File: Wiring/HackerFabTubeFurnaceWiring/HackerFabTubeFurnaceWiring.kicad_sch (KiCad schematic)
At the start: 11 parts

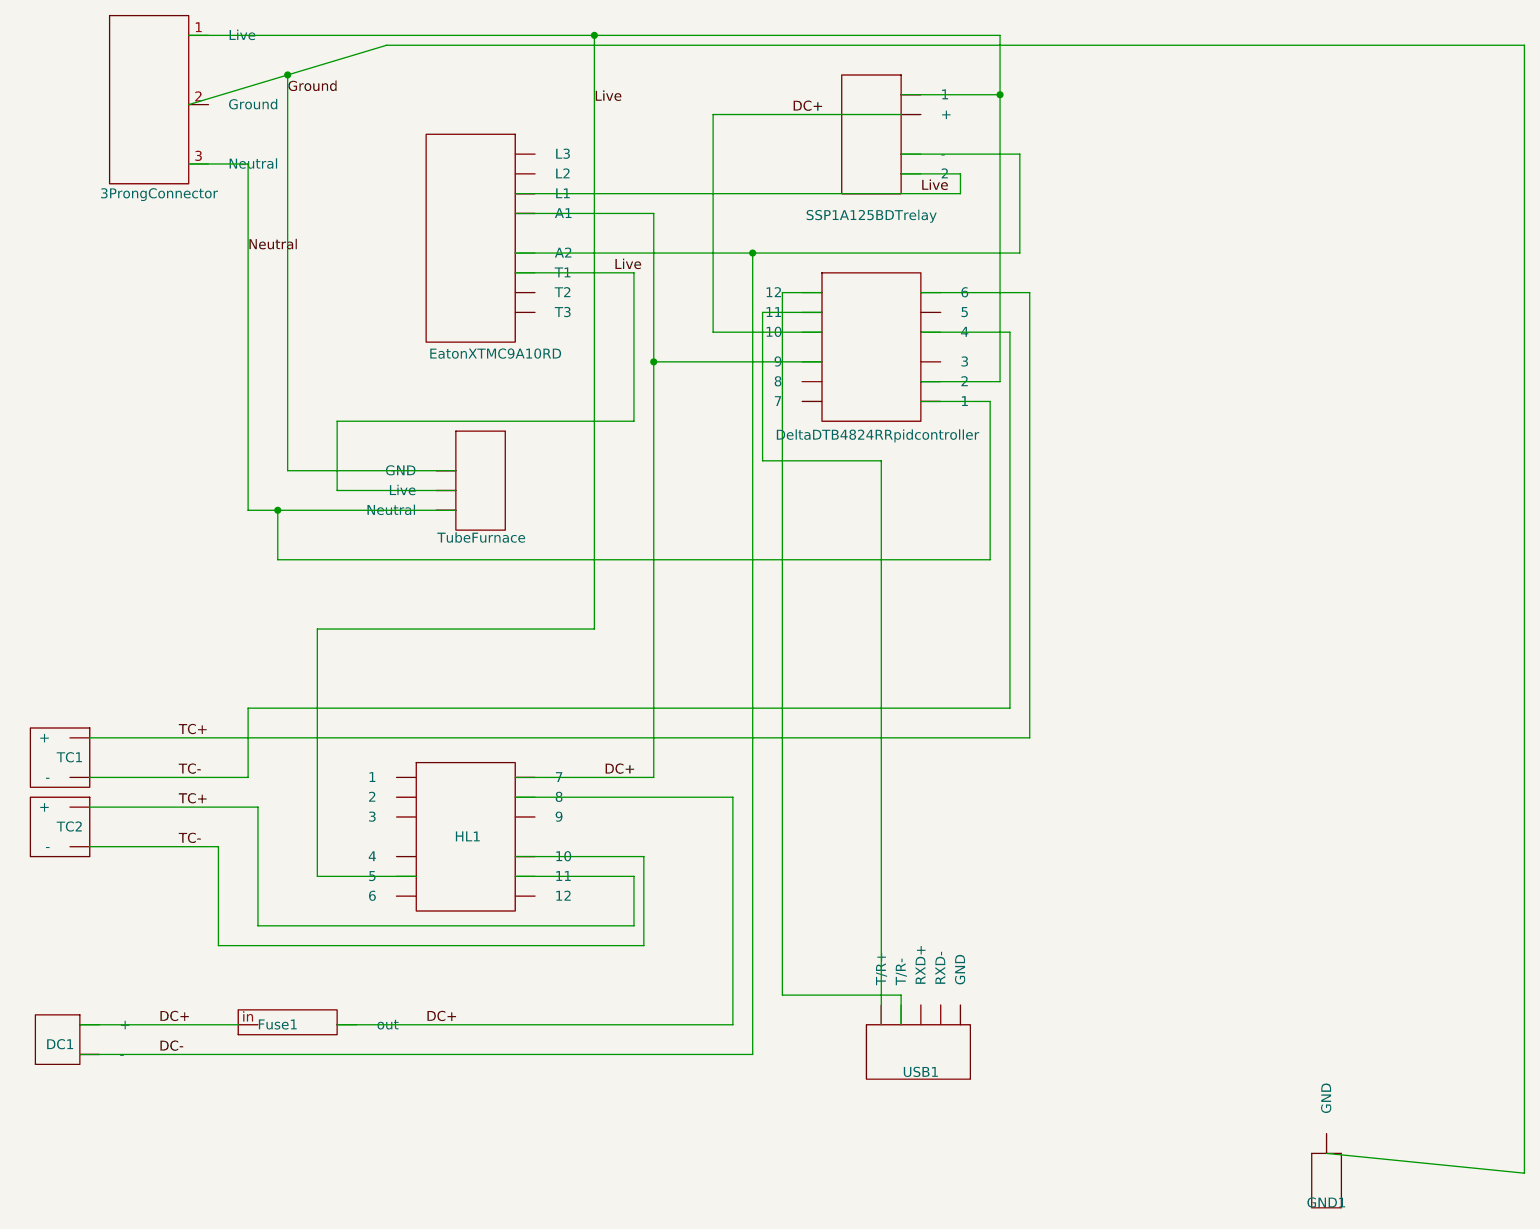
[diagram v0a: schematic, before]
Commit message: Adjustments to Schematic
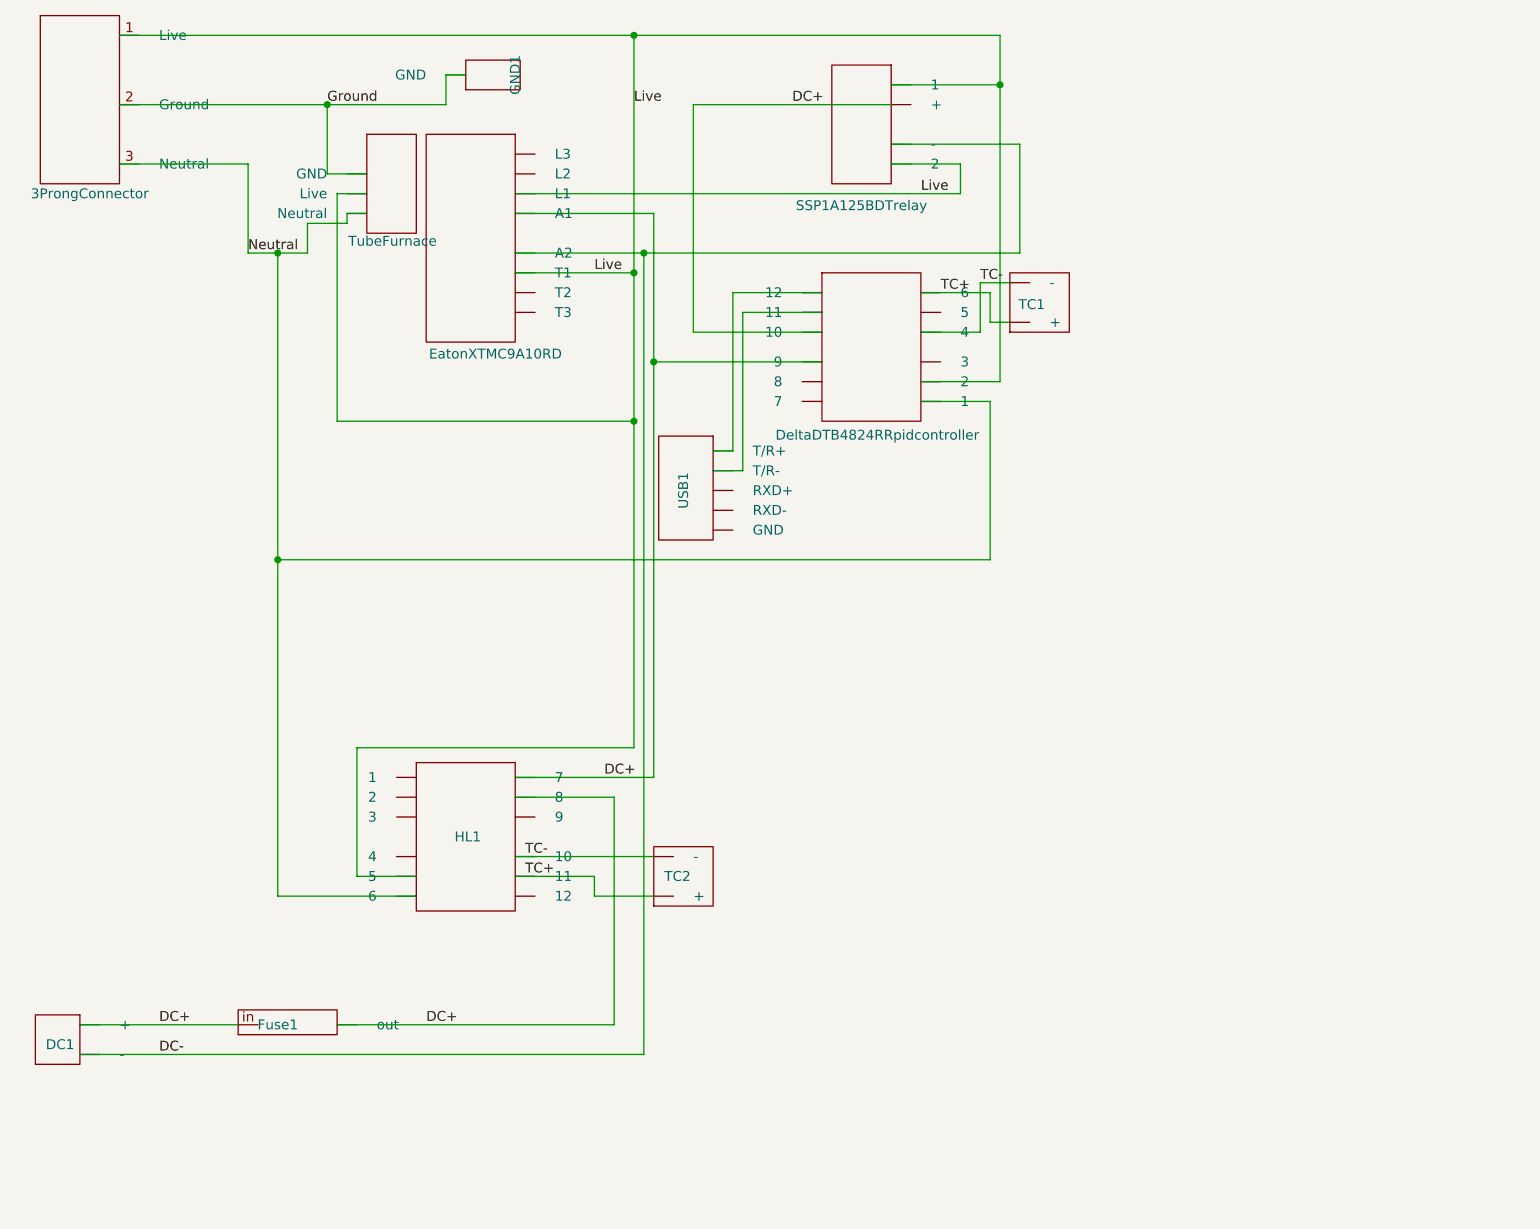
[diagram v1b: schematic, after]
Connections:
- net Neutral: now also HL1. (12)
- net at USB1. (GND): now also DeltaDTB4824RRpidcontroller. (1)
- new net: DeltaDTB4824RRpidcontroller. (1), USB1. (GND)
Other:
- moved on the sheet: GND1, SSP1A125BDTrelay, TC1, TC2, TubeFurnace, USB1
